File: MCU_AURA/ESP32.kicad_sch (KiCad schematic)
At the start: 14 parts, among them U200 ESP32-S3-WROOM-1, U201 USBLC6-2SC6

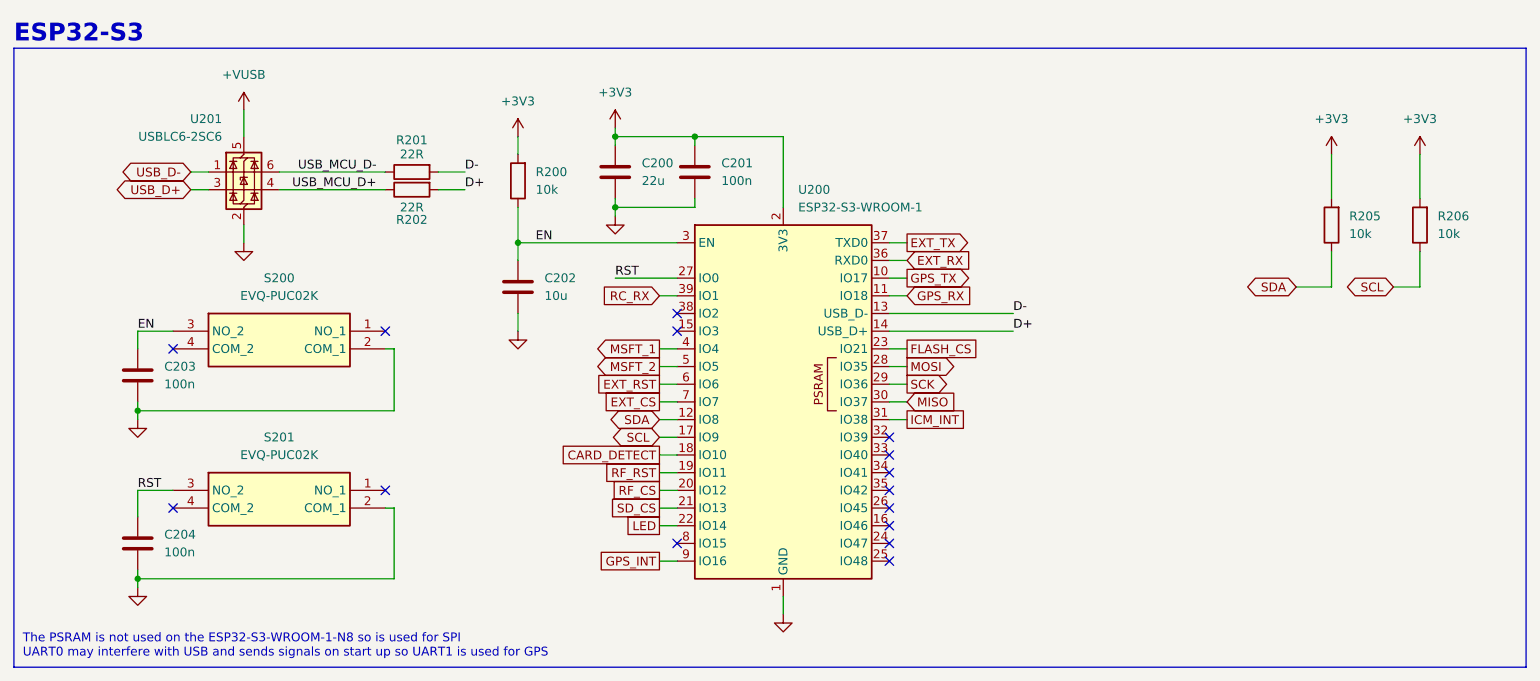
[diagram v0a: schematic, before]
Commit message: Second Iteration MCU
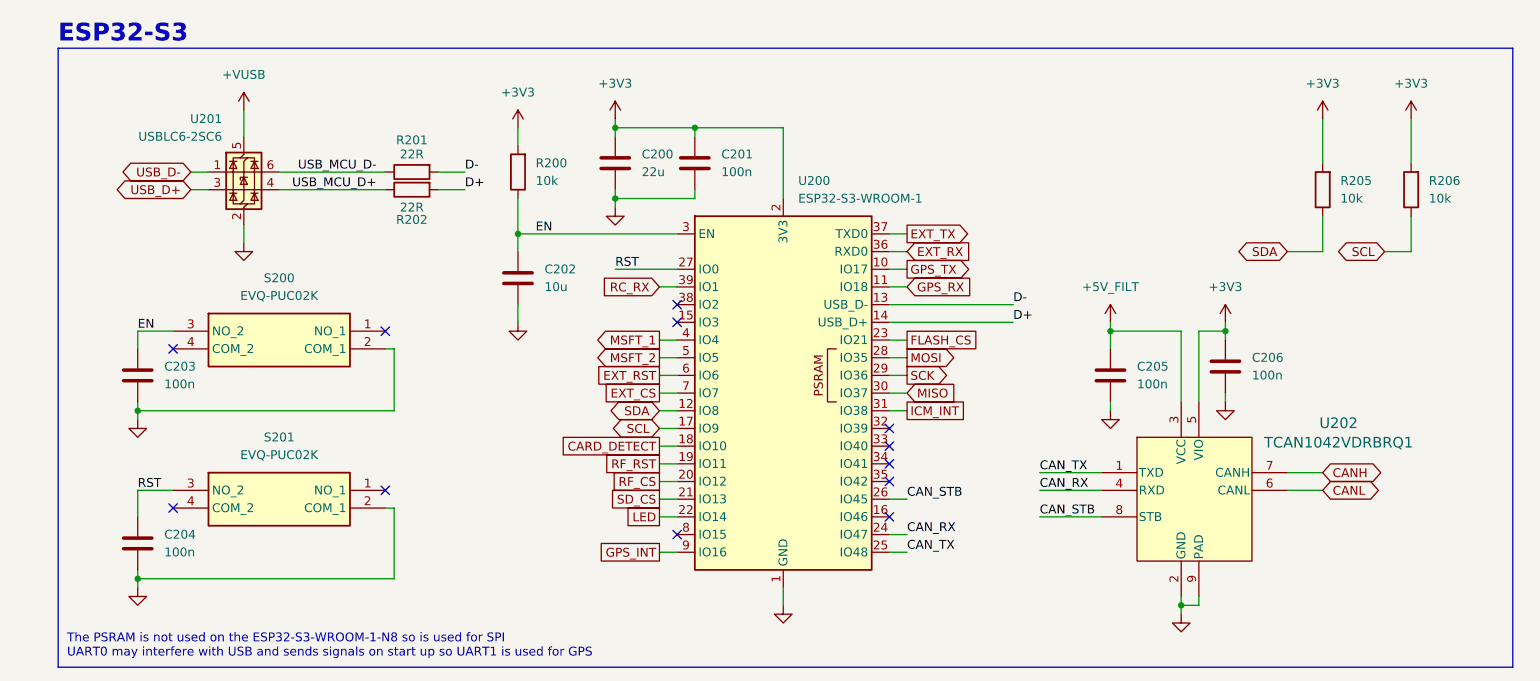
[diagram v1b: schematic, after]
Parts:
- added C205, C206: 100n, Capacitor_SMD:C_0402_1005Metric, symbol Device:C
- added U202: TCAN1042VDRBRQ1, TCAN1042VDRBRQ1:DRB0008F, symbol TCAN1042VDRBRQ1:TCAN1042VDRBRQ1
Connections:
- net +3V3: now also C206.1, U202.5 (VIO)
- net GND: now also C205.2, C206.2, U202.2 (GND), U202.9 (PAD)
- net CAN_RX: now reaches U200.24 (IO47)
- net CAN_RX: now also U202.4 (RXD)
- net CAN_TX: now reaches U200.25 (IO48)
- net CAN_TX: now also U202.1 (TXD)
- net CAN_STB: now reaches U200.26 (IO45)
- net CAN_STB: now also U202.8 (STB)
- new net +5V_FILT: C205.1, U202.3 (VCC)
- new net CANH: U202.7 (CANH)
- new net CANL: U202.6 (CANL)
- no-connect marks 15 -> 12
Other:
- moved on the sheet: C200, C201, C202, R200, R205, R206, U200
